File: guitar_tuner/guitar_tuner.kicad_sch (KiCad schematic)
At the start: 8 parts, among them SW1 Reset, SW2 Boot, U1 ESP32-S2-SOLO

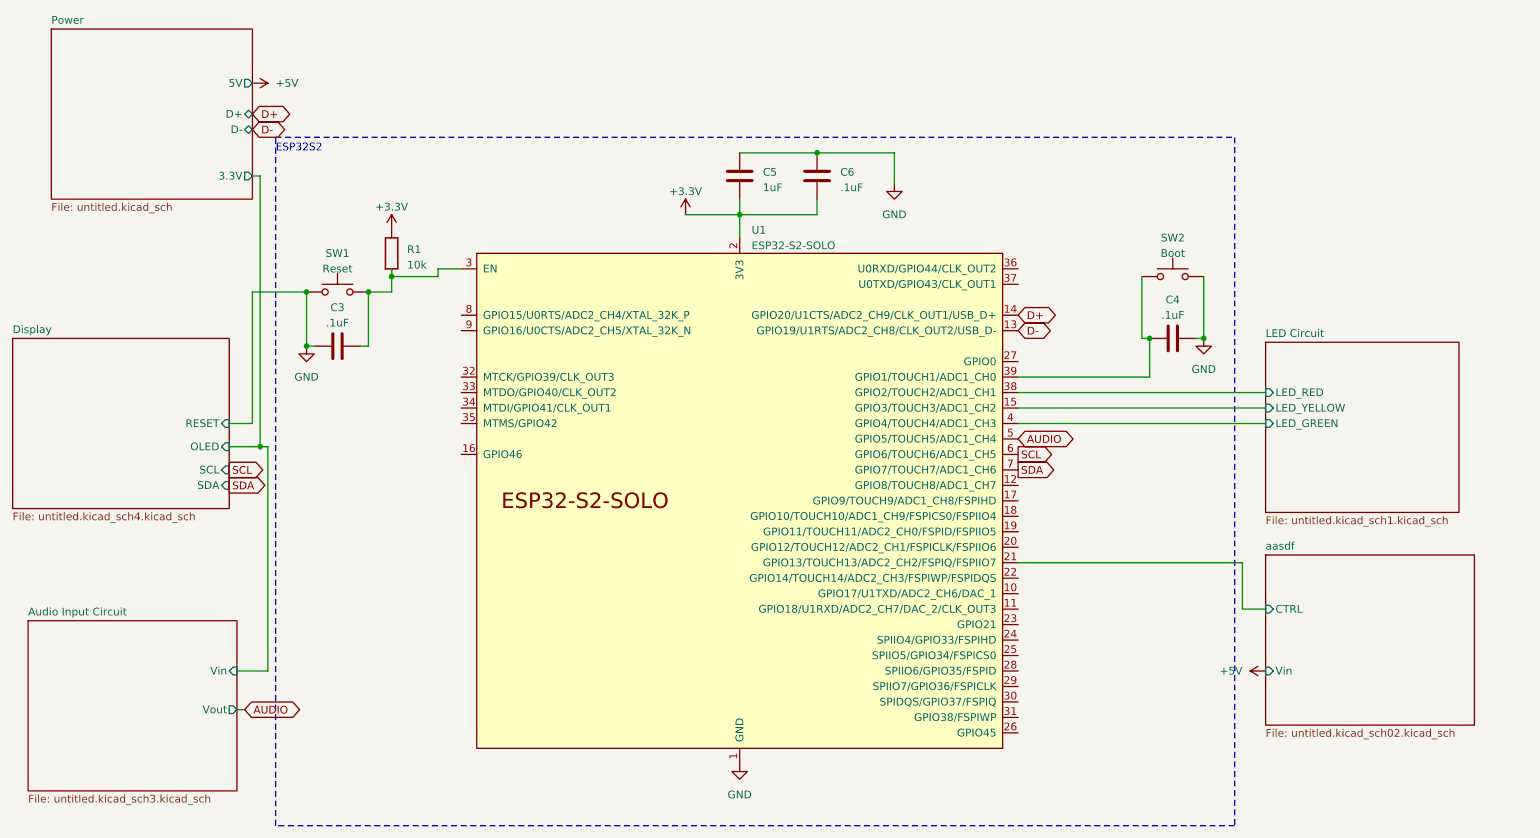
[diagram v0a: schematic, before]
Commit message: Screen
New Screen
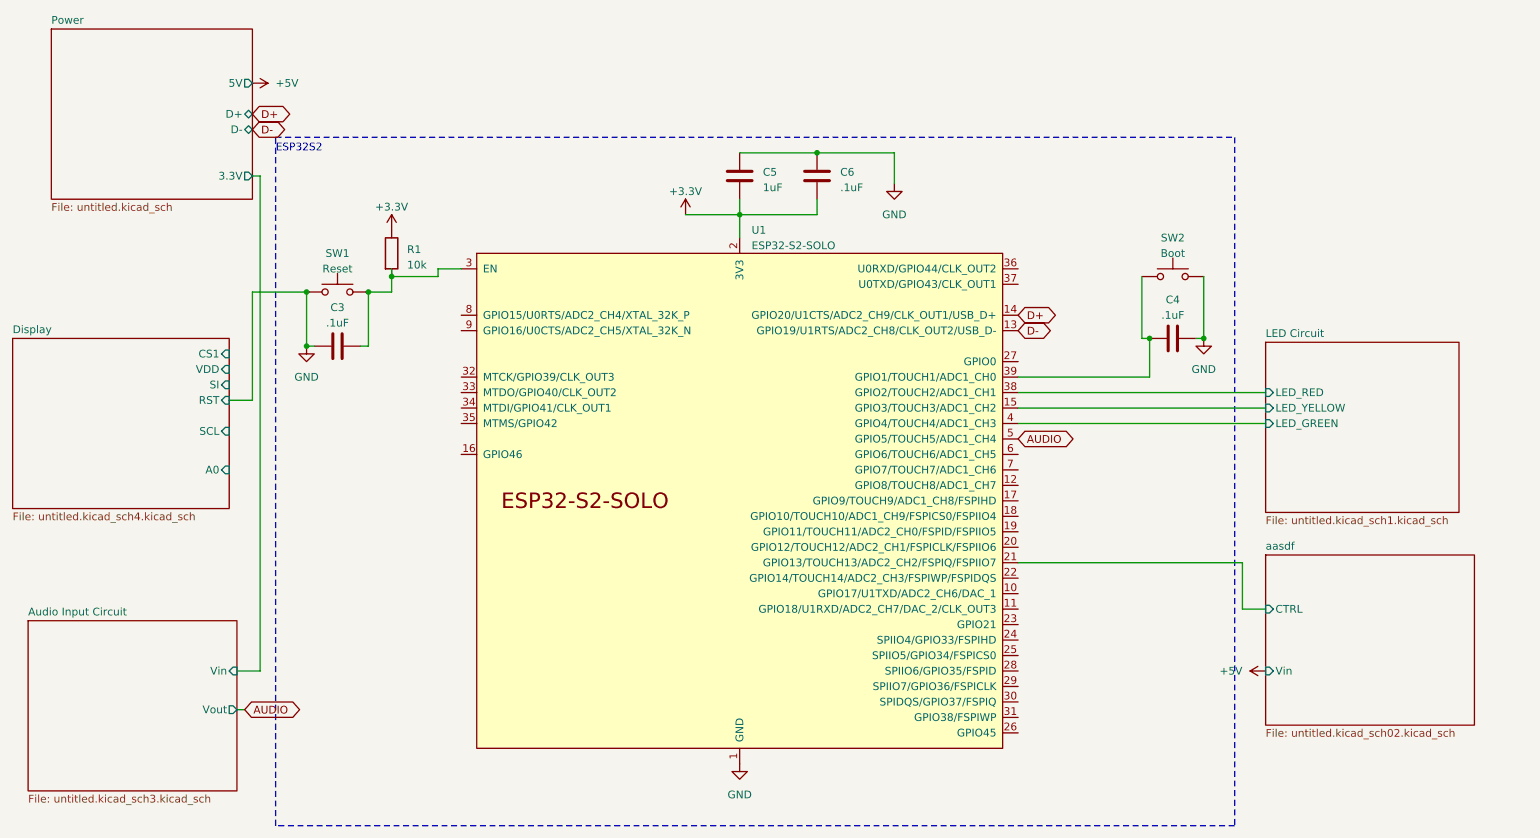
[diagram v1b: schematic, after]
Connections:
- net SCL: no longer names the net of U1.6 (GPIO6/TOUCH6/ADC1_CH5)
- net SDA: no longer names the net of U1.7 (GPIO7/TOUCH7/ADC1_CH6)
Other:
- sheet Display ports: added A0, CS1, RST, SI, VDD; removed OLED, RESET, SDA
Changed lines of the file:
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@@
-	)
-	(junction
-		(at 58.42 91.44)
-		(diameter 0)
-		(color 0 0 0 0)
 	)
 	(junction
@@
 	(wire
 		(pts
-			(xy 57.15 87.63) (xy 57.15 66.04)
-		)
-		(stroke
-			(width 0)
-			(type default)
-		)
-	)
-	(wire
-		(pts
-			(xy 53.34 87.63) (xy 57.15 87.63)
-		)
-		(stroke
-			(width 0)
-			(type default)
-		)
-	)
-	(wire
-		(pts
 			(xy 76.2 66.04) (xy 76.2 74.93)
 		)
@@
 	(wire
 		(pts
-			(xy 59.69 128.27) (xy 54.61 128.27)
+			(xy 58.42 128.27) (xy 54.61 128.27)
 		)
 		(stroke
@@
 	(wire
 		(pts
+			(xy 57.15 83.82) (xy 57.15 66.04)
+		)
+		(stroke
+			(width 0)
+			(type default)
+		)
+	)
+	(wire
+		(pts
 			(xy 182.88 87.63) (xy 223.52 87.63)
 		)
@@
 	(wire
 		(pts
-			(xy 58.42 91.44) (xy 59.69 91.44)
-		)
-		(stroke
-			(width 0)
-			(type default)
-		)
-	)
-	(wire
-		(pts
 			(xy 57.15 66.04) (xy 66.04 66.04)
 		)
@@
 	(wire
 		(pts
-			(xy 59.69 91.44) (xy 59.69 128.27)
+			(xy 58.42 46.99) (xy 58.42 128.27)
 		)
 		(stroke
@@
 	(wire
 		(pts
-			(xy 53.34 91.44) (xy 58.42 91.44)
-		)
-		(stroke
-			(width 0)
-			(type default)
-		)
-	)
-	(wire
-		(pts
 			(xy 213.36 63.5) (xy 213.36 73.66)
 		)
@@
 	(wire
 		(pts
-			(xy 58.42 91.44) (xy 58.42 46.99)
-		)
-		(stroke
-			(width 0)
-			(type default)
-		)
-	)
-	(wire
-		(pts
 			(xy 128.27 53.34) (xy 137.16 53.34)
+		)
+		(stroke
+			(width 0)
+			(type default)
+		)
+	)
+	(wire
+		(pts
+			(xy 53.34 83.82) (xy 57.15 83.82)
 		)
 		(stroke
@@
 		)
 	)
-	(global_label "SCL"
-		(shape output)
-		(at 53.34 95.25 0)
+	(global_label "D-"
+		(shape bidirectional)
+		(at 57.15 39.37 0)
 		(fields_autoplaced yes)
 		(effects
@@
 		)
 		(property "Intersheetrefs" "${INTERSHEET_REFS}"
-			(at 59.8328 95.25 0)
-			(effects
-				(font
-					(size 1.27 1.27)
-				)
-				(justify left)
-				(hide yes)
-			)
-		)
-	)
-	(global_label "SCL"
-		(shape output)
-		(at 182.88 92.71 0)
+			(at 64.0889 39.37 0)
+			(effects
+				(font
+					(size 1.27 1.27)
+				)
+				(justify left)
+				(hide yes)
+			)
+		)
+	)
+	(global_label "AUDIO"
+		(shape bidirectional)
+		(at 55.88 134.62 0)
 		(fields_autoplaced yes)
 		(effects
@@
 		)
 		(property "Intersheetrefs" "${INTERSHEET_REFS}"
-			(at 189.3728 92.71 0)
-			(effects
-				(font
-					(size 1.27 1.27)
-				)
-				(justify left)
-				(hide yes)
-			)
-		)
-	)
-	(global_label "SDA"
-		(shape output)
-		(at 182.88 95.25 0)
-		(fields_autoplaced yes)
-		(effects
-			(font
-				(size 1.27 1.27)
-			)
-			(justify left)
-		)
-		(property "Intersheetrefs" "${INTERSHEET_REFS}"
-			(at 189.4333 95.25 0)
-			(effects
-				(font
-					(size 1.27 1.27)
-				)
-				(justify left)
-				(hide yes)
-			)
-		)
-	)
-	(global_label "D-"
-		(shape bidirectional)
-		(at 57.15 39.37 0)
-		(fields_autoplaced yes)
-		(effects
-			(font
-				(size 1.27 1.27)
-			)
-			(justify left)
-		)
-		(property "Intersheetrefs" "${INTERSHEET_REFS}"
-			(at 64.0889 39.37 0)
-			(effects
-				(font
-					(size 1.27 1.27)
-				)
-				(justify left)
-				(hide yes)
-			)
-		)
-	)
-	(global_label "AUDIO"
-		(shape bidirectional)
-		(at 55.88 134.62 0)
-		(fields_autoplaced yes)
-		(effects
-			(font
-				(size 1.27 1.27)
-			)
-			(justify left)
-		)
-		(property "Intersheetrefs" "${INTERSHEET_REFS}"
 			(at 65.6009 134.62 0)
-			(effects
-				(font
-					(size 1.27 1.27)
-				)
-				(justify left)
-				(hide yes)
-			)
-		)
-	)
-	(global_label "SDA"
-		(shape output)
-		(at 53.34 97.79 0)
-		(fields_autoplaced yes)
-		(effects
-			(font
-				(size 1.27 1.27)
-			)
-			(justify left)
-		)
-		(property "Intersheetrefs" "${INTERSHEET_REFS}"
-			(at 59.8933 97.79 0)
 			(effects
 				(font
@@
 			)
 		)
-		(pin "OLED" input
-			(at 53.34 91.44 0)
+		(pin "CS1" input
+			(at 53.34 76.2 0)
 			(effects
 				(font
@@
 			)
 		)
-		(pin "RESET" input
-			(at 53.34 87.63 0)
+		(pin "VDD" input
+			(at 53.34 78.74 0)
 			(effects
 				(font
@@
 			)
 		)
+		(pin "SI" input
+			(at 53.34 81.28 0)
+			(effects
+				(font
+					(size 1.27 1.27)
+				)
+				(justify right)
+			)
+		)
+		(pin "RST" input
+			(at 53.34 83.82 0)
+			(effects
+				(font
+					(size 1.27 1.27)
+				)
+				(justify right)
+			)
+		)
+		(pin "A0" input
+			(at 53.34 95.25 0)
+			(effects
+				(font
+					(size 1.27 1.27)
+				)
+				(justify right)
+			)
+		)
 		(pin "SCL" input
-			(at 53.34 95.25 0)
-			(effects
-				(font
-					(size 1.27 1.27)
-				)
-				(justify right)
-			)
-		)
-		(pin "SDA" input
-			(at 53.34 97.79 0)
-			(effects
-				(font
+			(at 53.34 88.9 0)
+			(effects
+				(font
